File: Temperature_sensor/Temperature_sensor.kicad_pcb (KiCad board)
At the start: 4 copper layers, 41 x 55.2 mm, 35 parts, among them IC1 TC7660, J1 BAT_GND, J2 BAT_3.7V, SW1 SW_Push, SW2 SW_Push, SW3 SW_Push, U1 TP4056, U2 ESP32-S3-ZERO, U3 LM35-LP, U4 DM-OLED096-636

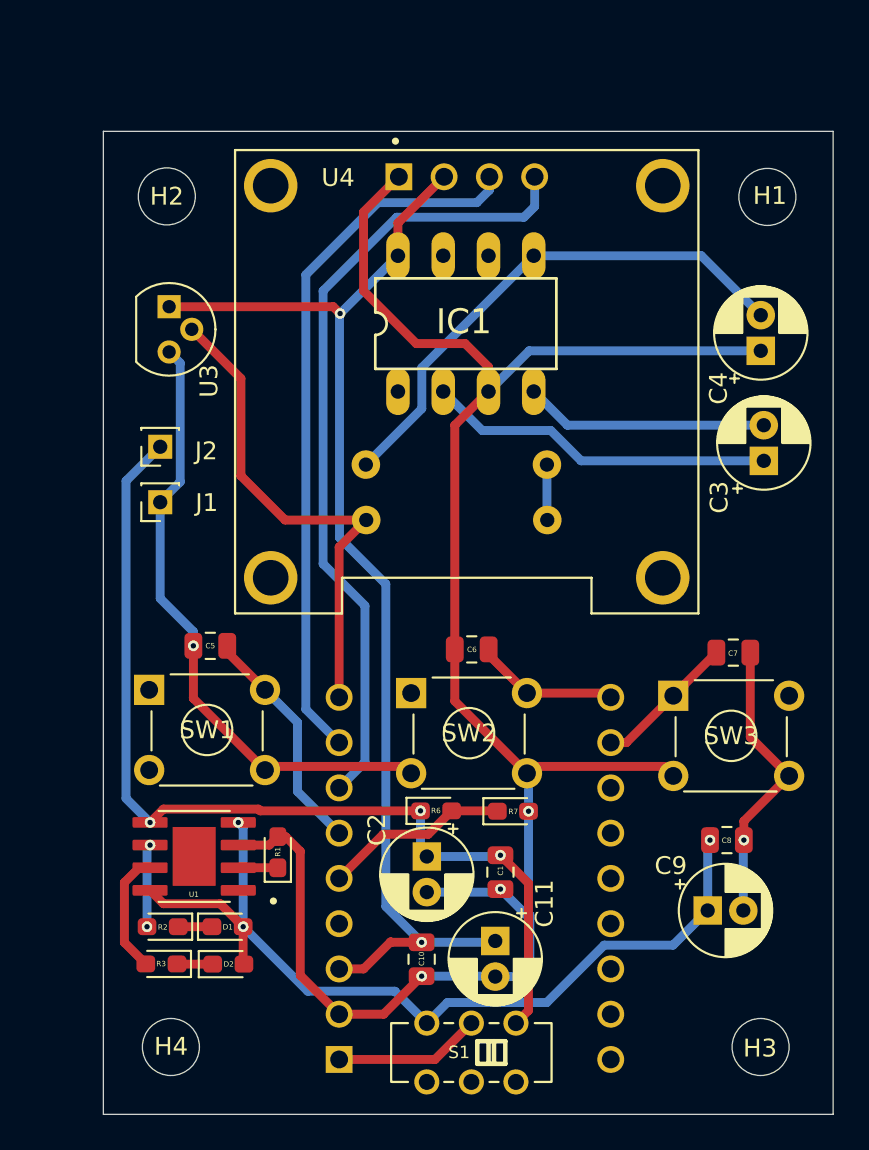
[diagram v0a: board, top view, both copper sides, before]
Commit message: final
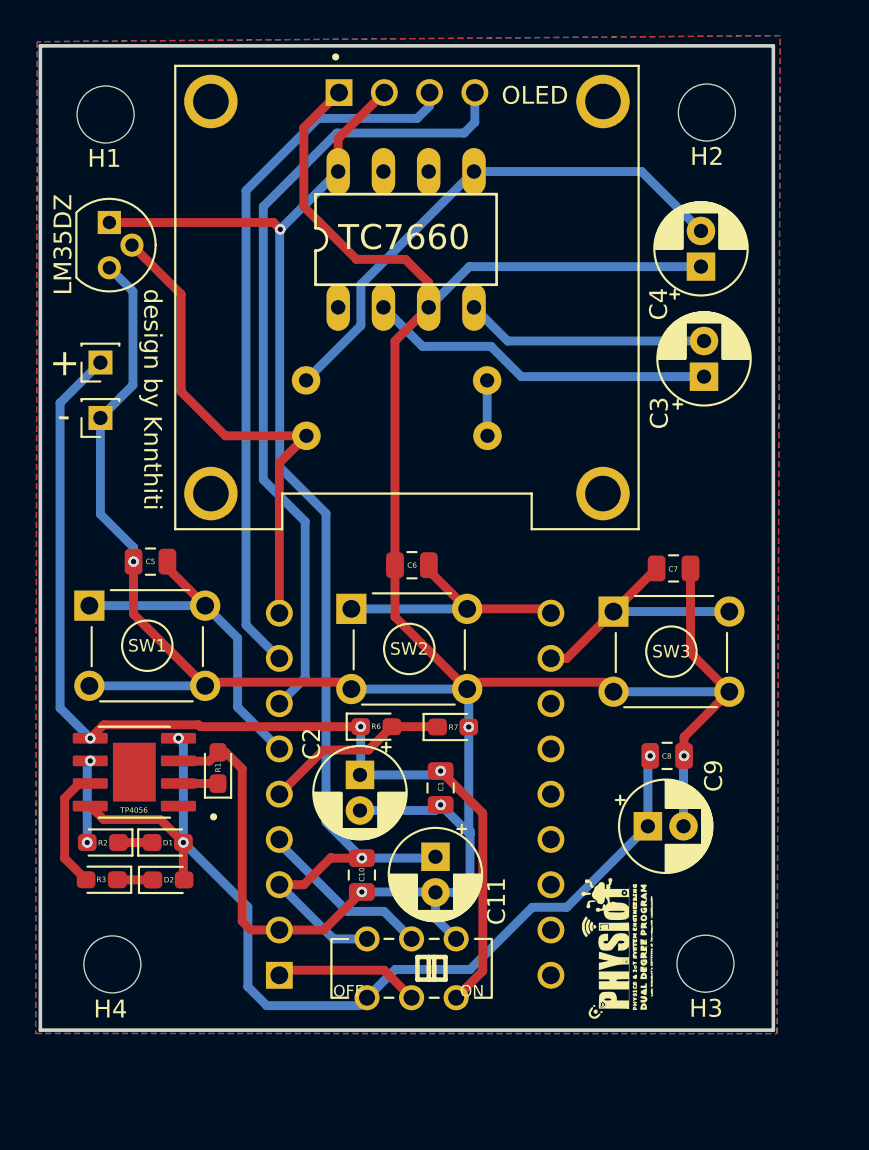
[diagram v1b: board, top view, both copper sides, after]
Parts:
- added G***: LOGO, logo:physic_iote_A95_50, F.Cu at (153.1, 108.2)
- added G***: LOGO, logo:KMITL, F.Cu at (132.1, 72.8)
- added G***: LOGO, logo:ichika_137_200, F.Cu at (153.9, 71.6)
- added G***: LOGO, logo:ROBOT, F.Cu at (157.6, 96.0)
- added G***: LOGO, logo:IERL, F.Cu at (128.7, 100.6)
- added G***: LOGO, logo:iote, F.Cu at (143.3, 81.3)
- OFF                   ON: renamed from S1
- moved H1 37.4 mm to (125.9, 60.7)
- moved H2 30.7 mm to (159.6, 60.6)
- moved C2 5.92 mm to (140.2, 97.8)
- moved D2 5.79 mm to (129.4, 103.6)
- moved R1 5.79 mm to (132.2, 97.4)
- moved R5 5.79 mm to (147.3, 75.6)
- moved R7 5.79 mm to (145.4, 95.1)
- moved SW1 5.79 mm to (125.0, 88.3)
- moved SW3 5.79 mm to (154.4, 88.6)
- moved esp32s3zero 5.79 mm to (143.3, 98.8)
- moved C10 5.79 mm to (140.3, 103.4)
- moved C4 5.79 mm to (159.3, 69.2)
- moved C6 5.79 mm to (143.1, 86.0)
- moved C7 5.79 mm to (157.8, 86.2)
- moved OLED 5.79 mm to (142.8, 71.0)
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- renumbered J2 to +, J1 to -, U3 to LM35DZ, U4 to OLED, IC1 to TC7660, U1 to TP4056, U2 to esp32s3zero
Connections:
- OFF                   ON pad 4: BAT -> 0
- OFF                   ON pad 5: Net-(S1-Pad2) -> GP1
- OFF                   ON pad 6: 5V -> 3.3V
- esp32s3zero pad 1: unconnected-(U2-GP1-Pad1) -> GP1
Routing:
- net GP1: track 0.00 -> 9.85 mm
- net 3.3V: track 66.6 -> 72.8 mm
- net 0: track 180.5 -> 185.6 mm
- net Net-(S1-Pad2): track 11.6 -> 8.51 mm
- net BAT: track 58.5 -> 61.0 mm
- net 5V: track 52.4 -> 54.8 mm
- added copper zone on B.Cu, net 0
- added copper zone on F.Cu, net 0
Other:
- board size 41 x 55.2 mm -> 41.1 x 55.2 mm
- copper layers 4 -> 2
- board text added: "design by Knnthiti"
